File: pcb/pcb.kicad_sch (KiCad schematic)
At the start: 2 parts

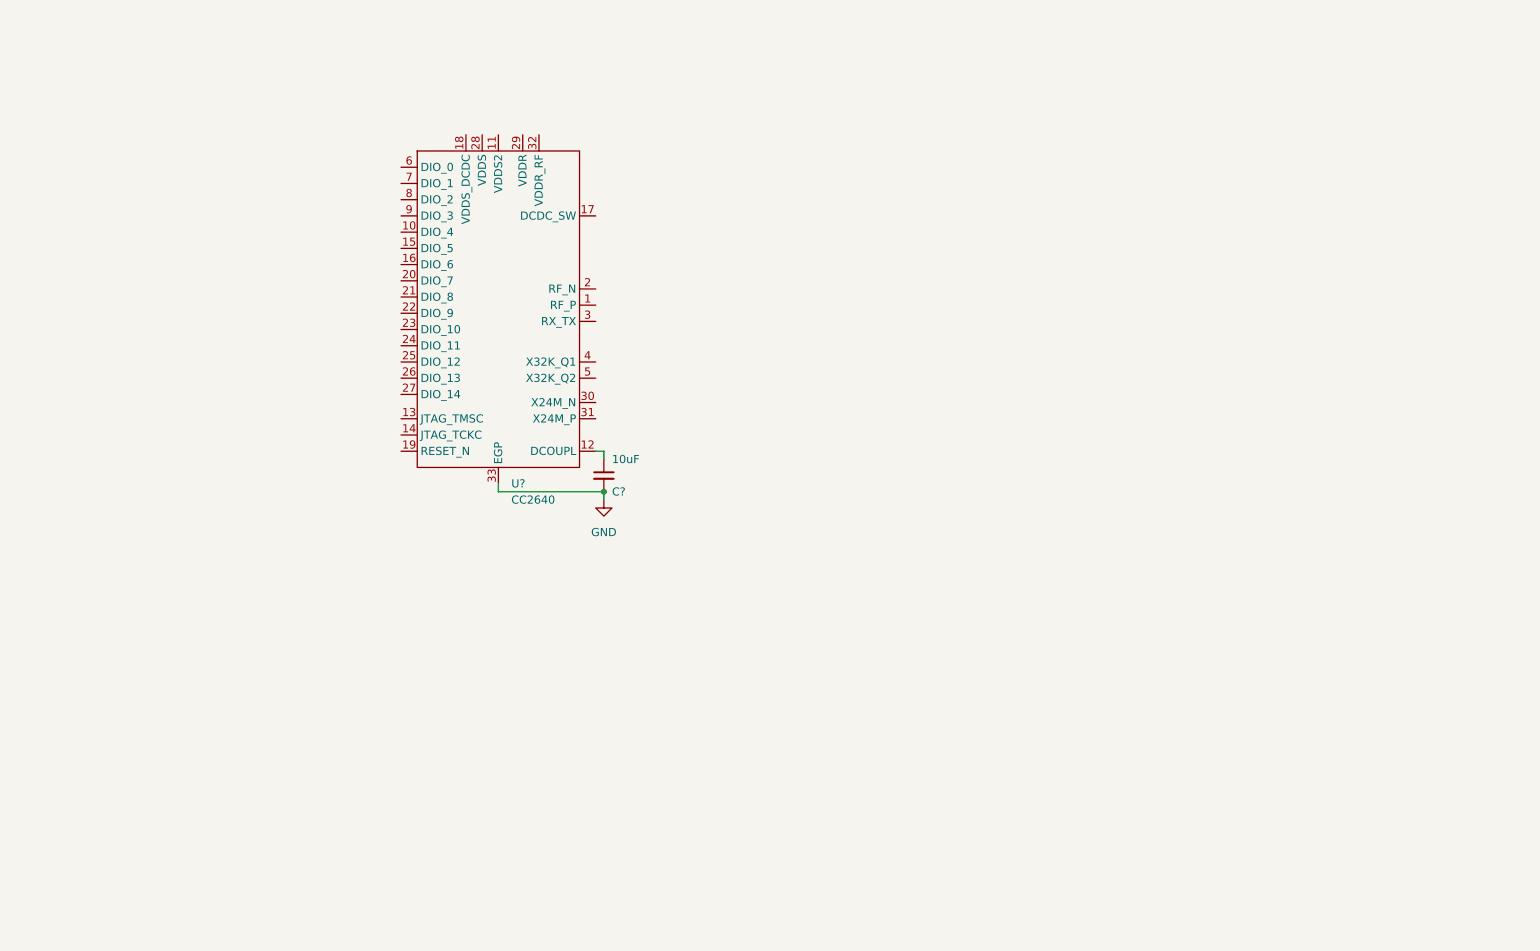
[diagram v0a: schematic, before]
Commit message: schematic
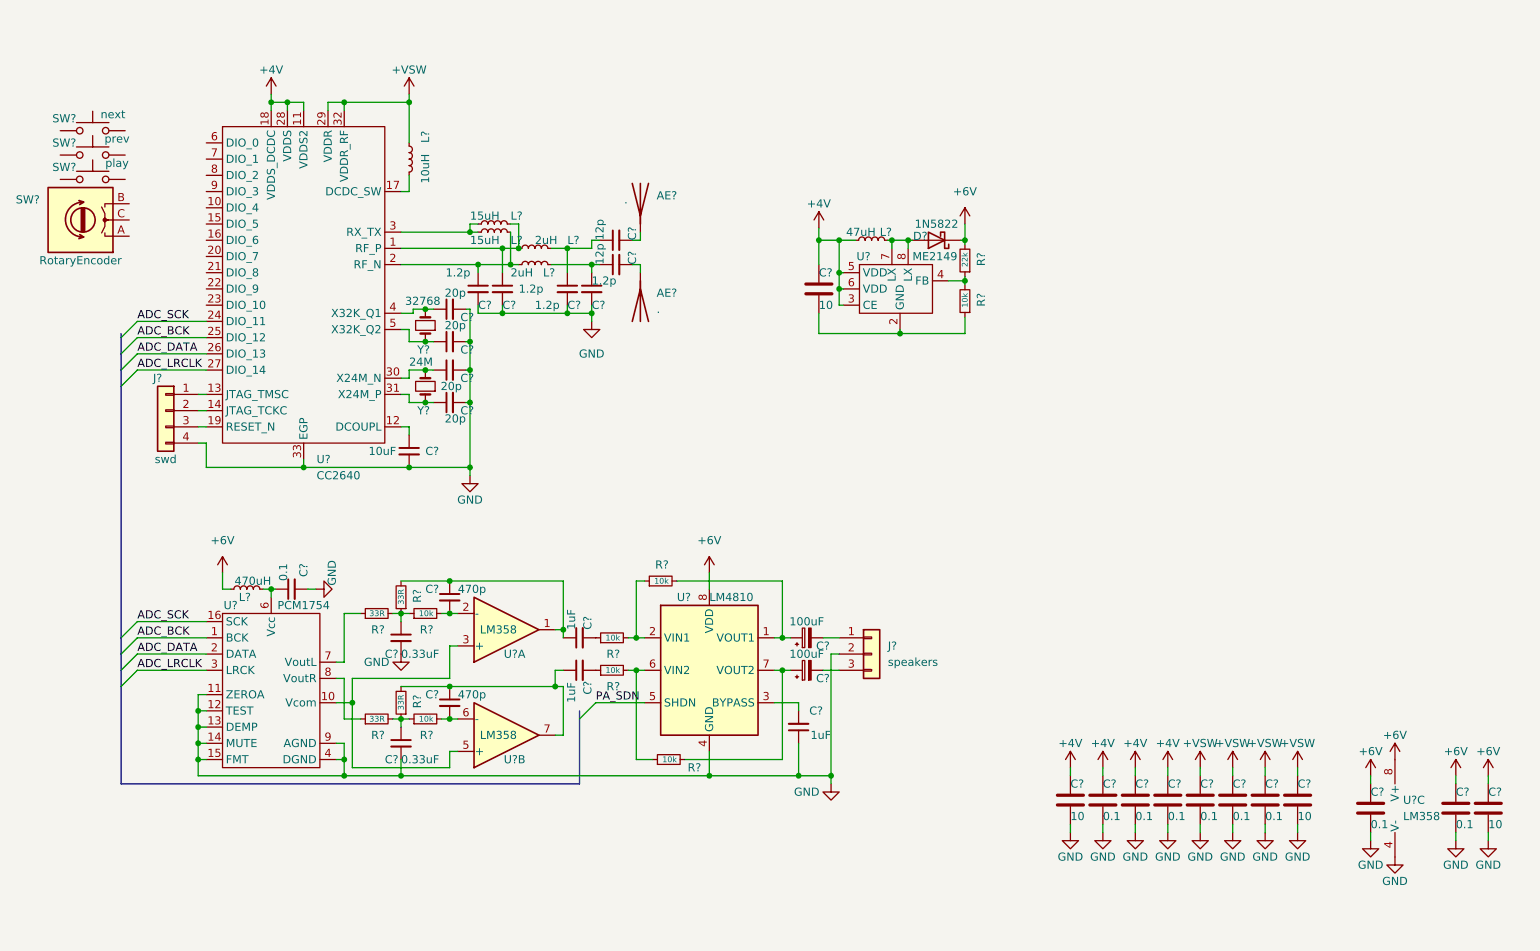
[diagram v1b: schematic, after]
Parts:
- added AE? (x2): ., symbol Device:Antenna
- added C? (x4): 1.2p, symbol Device:C_Small
- added C? (x2): 470p, symbol Device:C_Small
- added C? (x4): 20p, symbol Device:C_Small
- added C? (x8): 0.1, symbol Device:C
- added C? (x4): 10, symbol Device:C
- added C? (x2): 100uF, symbol Device:C_Polarized_Small
- added C? (x2): 12p, symbol Device:C_Small
- added C?: 0.1, symbol Device:C_Small
- added C? (x3): 1uF, symbol Device:C_Small
- added C? (x2): 0.33uF, symbol Device:C_Small
- added D?: 1N5822, symbol Device:D_Schottky
- added J?: speakers, symbol Connector_Generic:Conn_01x03
- added J?: swd, symbol Connector_Generic:Conn_01x04
- added L? (x2): 2uH, symbol Device:L_Small
- added L?: 47uH, symbol Device:L_Small
- added L? (x2): 15uH, symbol Device:L_Small
- added L?: 10uH, symbol Device:L_Small
- added L?: 470uH, symbol Device:L_Small
- added R? (x4): 33R, symbol Device:R_Small
- added R? (x7): 10k, symbol Device:R_Small
- added R?: 22k, symbol Device:R_Small
- added SW?: next, symbol Switch:SW_Push
- added SW?: play, symbol Switch:SW_Push
- added SW?: RotaryEncoder, symbol Device:RotaryEncoder
- added SW?: prev, symbol Switch:SW_Push
- added U? (x3): LM358, symbol Amplifier_Operational:LM358
- added U?: LM4810, Package_SO:TSSOP-8_3x3mm_P0.65mm, symbol Amplifier_Audio:LM4810
- added U?: PCM1754, symbol local:PCM1754
- added U?: ME2149, symbol local:ME2149
- added Y?: 24M, symbol Device:Crystal_Small
- added Y?: 32768, symbol Device:Crystal_Small
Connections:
- net GND: now also C?.1, C?.2, C?.2, C?.2, C?.2, C?.2, C?.2, C?.2, C?.2, C?.2, C?.2, C?.2, C?.2, C?.2, C?.2, C?.2, C?.2, C?.2, C?.2, C?.2, C?.2, C?.2, C?.2, J?.2 (Pin_2), J?.4 (Pin_4), U?.11 (ZEROA), U?.12 (TEST), U?.13 (DEMP), U?.14 (MUTE), U?.15 (FMT), U?.4 (DGND), U?.4 (GND), U?.4 (V-), U?.9 (AGND)
- net at U?.1 (RF_P): now also C?.1, L?.1, L?.2
- net +4V: now reaches U?.11 (VDDS2)
- net +4V: now also U?.18 (VDDS_DCDC), U?.28 (VDDS), C?.1, C?.1, C?.1, C?.1, C?.1, L?.1, U?.3 (CE), U?.5 (VDD), U?.6 (VDD)
- net at U?.13 (JTAG_TMSC): now also J?.1 (Pin_1)
- net at U?.14 (JTAG_TCKC): now also J?.2 (Pin_2)
- net at U?.17 (DCDC_SW): now also L?.2
- net at U?.19 (RESET_N): now also J?.3 (Pin_3)
- net at U?.2 (RF_N): now also C?.1, L?.1, L?.2
- net ADC_SCK: now reaches U?.24 (DIO_11)
- net ADC_SCK: now also U?.16 (SCK)
- net ADC_BCK: now reaches U?.25 (DIO_12)
- net ADC_BCK: now also U?.1 (BCK)
- net ADC_DATA: now reaches U?.26 (DIO_13)
- net ADC_DATA: now also U?.2 (DATA)
- net ADC_LRCLK: now reaches U?.27 (DIO_14)
- net ADC_LRCLK: now also U?.3 (LRCK)
- net +VSW: now reaches U?.29 (VDDR)
- net +VSW: now also U?.32 (VDDR_RF), C?.1, C?.1, C?.1, C?.1, L?.1
- net at U?.3 (RX_TX): now also L?.2, L?.2
- net at U?.30 (X24M_N): now also C?.1, Y?.2
- net at U?.31 (X24M_P): now also C?.1, Y?.1
- net at U?.4 (X32K_Q1): now also C?.1, Y?.2
- net at U?.5 (X32K_Q2): now also C?.1, Y?.1
- new net: R?.1, U?.8 (VoutR)
- new net: C?.1, R?.1, R?.1, R?.2 (x2)
- new net: C?.1, C?.1, L?.1 (x2)
- new net: C?.1, C?.1, R?.2, U?.7
- new net: C?.2, R?.2, U?.6 (-)
- new net: C?.2, R?.2, U?.2 (-)
- new net: C?.1, C?.1, R?.2, U?.1
- new net: U?.10 (Vcom), U?.3 (+), U?.5 (+)
- new net: R?.1, R?.2, U?.2 (VIN1)
- new net: C?.1, R?.2, U?.1 (VOUT1)
- new net: D?.2 (A), L?.2, U?.7 (LX), U?.8 (LX)
- new net: R?.1, R?.2, U?.6 (VIN2)
- new net: C?.1, R?.2, U?.7 (VOUT2)
- new net: C?.2, R?.1, U?.2 (GND)
- new net: R?.1, R?.2, U?.4 (FB)
- new net: AE?.1 (A), C?.2 (x2)
- new net: C?.2, J?.3 (Pin_3)
- new net: C?.2, J?.1 (Pin_1)
- new net: C?.2, R?.1 (x2)
- new net: C?.1, L?.2, U?.6 (Vcc)
- new net: C?.2, U?.3 (BYPASS)
- new net: R?.1, U?.7 (VoutL)
- new net +6V: C?.1, C?.1, C?.1, D?.1 (K), L?.1, R?.2, U?.8 (V+), U?.8 (VDD)
- new net PA_SDN: U?.5 (SHDN)
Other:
- moved on the sheet: C?, U?

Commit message: schematic png
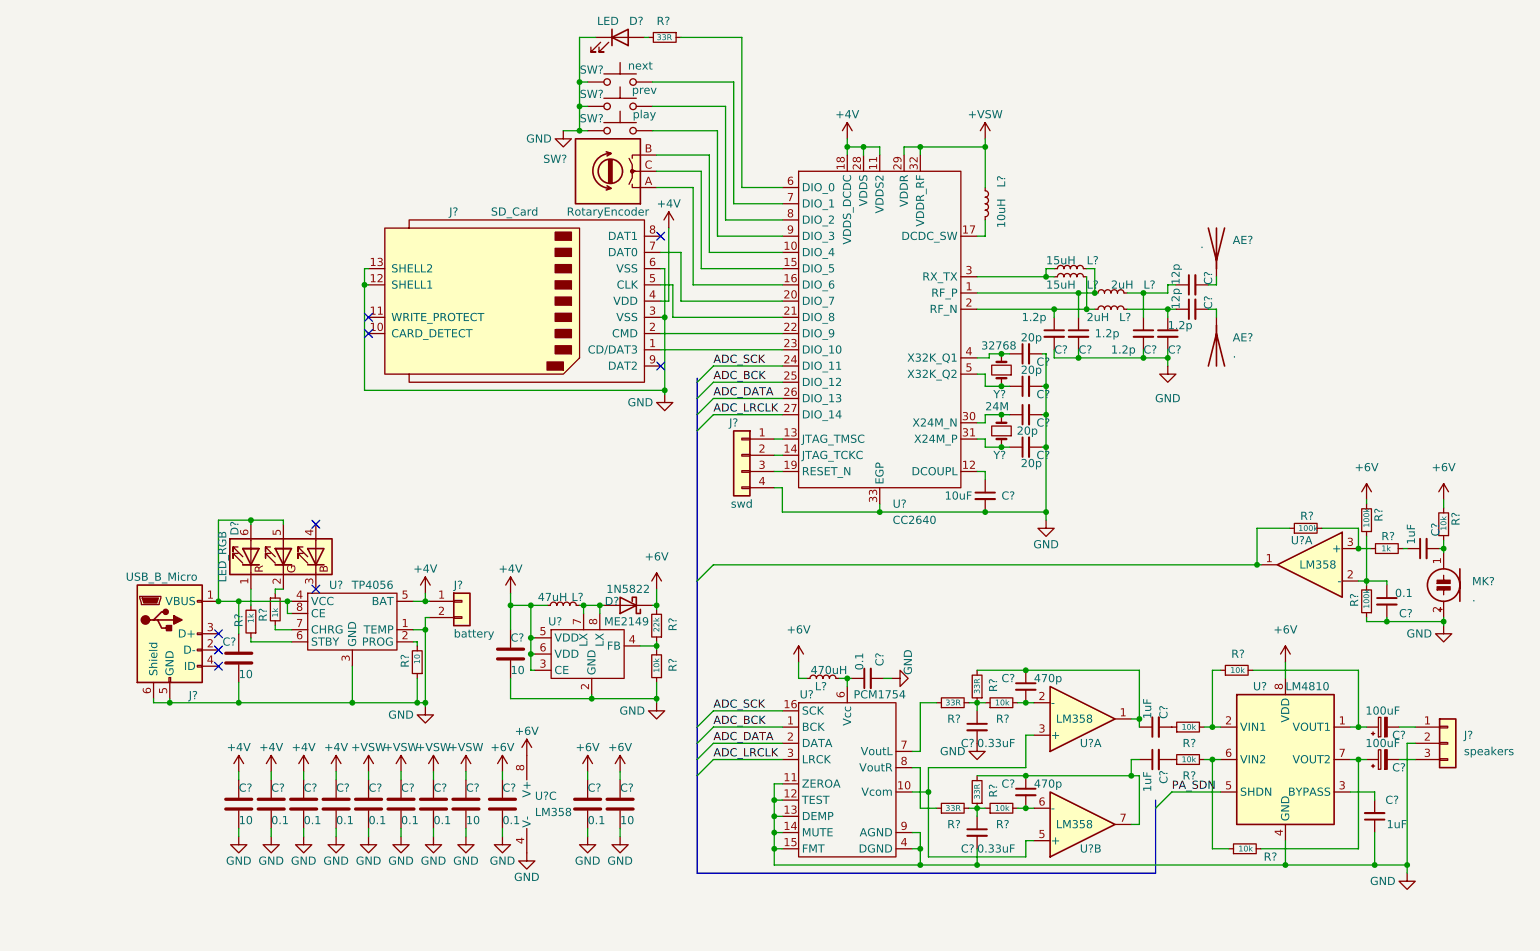
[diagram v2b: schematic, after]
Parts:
- added C?: 0.1, symbol Device:C_Small
- added C?: 10, symbol Device:C
- added C?: 1uF, symbol Device:C_Small
- added D?: LED, symbol Device:LED
- added D?: LED_RGB, symbol Device:LED_RGB
- added J?: SD_Card, symbol Connector:SD_Card
- added J?: USB_B_Micro, symbol Connector:USB_B_Micro
- added J?: battery, symbol Connector_Generic:Conn_01x02
- added MK?: ., symbol Device:Microphone_Condenser
- added R? (x3): 1k, symbol Device:R_Small
- added R? (x3): 100k, symbol Device:R_Small
- added R?: 10, symbol Device:R_Small
- added R?: 10k, symbol Device:R_Small
- added R?: 33R, symbol Device:R_Small
- added U?: TP4056, symbol local:TP4056
- added U?: LM358, symbol Amplifier_Operational:LM358
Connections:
- net +4V: now also J?.1 (Pin_1), J?.4 (VDD), U?.5 (BAT)
- net +6V: now also R?.2, R?.2
- net GND: now also C?.2, R?.1, SW?.1, SW?.1, SW?.1, U?.2 (GND), C?.2, C?.2, D?.1 (K), J?.12 (SHELL1), J?.13 (SHELL2), J?.2 (Pin_2), J?.3 (VSS), J?.5 (GND), J?.6 (Shield), J?.6 (VSS), MK?.2 (+), R?.1, R?.1, U?.1 (TEMP), U?.3 (GND)
- net at SW?.2: now also U?.7 (DIO_1)
- net at U?.10 (DIO_4): now also SW?.B
- net at U?.15 (DIO_5): now also SW?.C
- net at U?.16 (DIO_6): now also SW?.A
- net at U?.20 (DIO_7): now also J?.7 (DAT0)
- net at U?.21 (DIO_8): now also J?.5 (CLK)
- net at U?.22 (DIO_9): now also J?.2 (CMD)
- net at U?.23 (DIO_10): now also J?.1 (CD/DAT3)
- net at U?.6 (DIO_0): now also R?.1
- net at U?.8 (DIO_2): now also SW?.2
- net at U?.9 (DIO_3): now also SW?.2
- new net: R?.1, R?.2, U?.3 (+)
- new net: C?.1, R?.2
- new net: D?.2 (A), R?.2
- new net: C?.1, R?.1, R?.2, U?.2 (-)
- new net: R?.2, U?.2 (PROG)
- new net: C?.2, MK?.1 (-), R?.1
- new net: C?.1, D?.5 (GA), D?.6 (RA), J?.1 (VBUS), U?.4 (VCC), U?.8 (CE)
- new net: R?.1, U?.6 (STBY)
- new net: R?.2, U?.7 (CHRG)
- new net: D?.1 (RK), R?.2
- new net: D?.2 (GK), R?.1
- new net: R?.1, U?.1
- no-connect marks 0 -> 9
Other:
- moved on the sheet: AE?, C?, D?, J?, L?, R?, SW?, U?, U?A, U?B, U?C, Y?

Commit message: pcb footprints
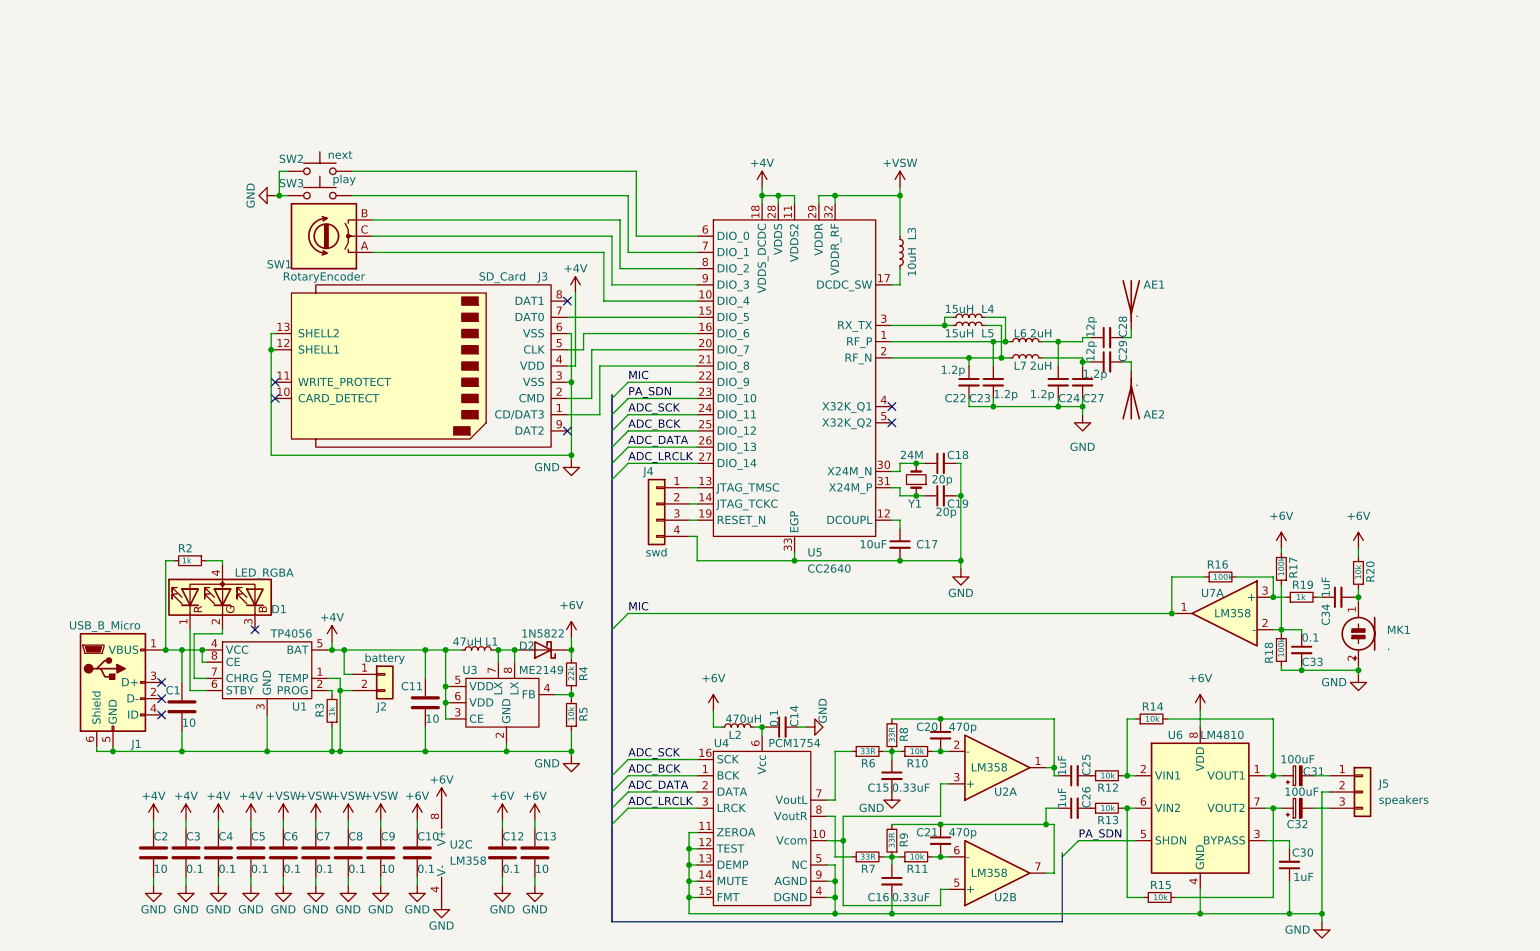
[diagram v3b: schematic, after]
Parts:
- removed C? (x2): 20p, symbol Device:C_Small
- removed D?: LED, symbol Device:LED
- removed D?: LED_RGB, symbol Device:LED_RGB
- removed R?: 1k, symbol Device:R_Small
- removed R?: 33R, symbol Device:R_Small
- removed SW?: prev, symbol Switch:SW_Push
- removed Y?: 32768, symbol Device:Crystal_Small
- added D1: LED_RGBA, LED_SMD:LED_Cree-PLCC4_3.2x2.8mm_CCW, symbol Device:LED_RGBA
- AE1, AE2: renamed from AE?; footprint (none) -> Connector_Wire:SolderWirePad_1x01_SMD_1x2mm
- C1, C11, C13, C17, C2, C25, C26, C30, C34, C9: renamed from C?; footprint (none) -> Capacitor_SMD:C_0805_2012Metric
- C10, C12, C14, C18, C19, C3, C33, C4, C5, C6, C7, C8: renamed from C?; footprint (none) -> Capacitor_SMD:C_0402_1005Metric
- C15, C16, C20, C21, C22, C23, C24, C27, C28, C29: renamed from C?; footprint (none) -> Capacitor_SMD:C_0603_1608Metric
- C31, C32: renamed from C?; footprint (none) -> Capacitor_Tantalum_SMD:CP_EIA-1608-08_AVX-J
- D2: renamed from D?; footprint (none) -> Diode_SMD:D_SMA
- J1: renamed from J?; footprint (none) -> Connector_USB:USB_Micro-B_Amphenol_10104110_Horizontal
- J2: renamed from J?; footprint (none) -> Connector_PinHeader_2.54mm:PinHeader_1x02_P2.54mm_Vertical
- J3: renamed from J?; footprint (none) -> Connector_Card:SD_Hirose_DM1AA_SF_PEJ82
- J4: renamed from J?; footprint (none) -> Connector_PinHeader_1.00mm:PinHeader_1x04_P1.00mm_Vertical_SMD_Pin1Left
- J5: renamed from J?; footprint (none) -> Connector_PinHeader_2.54mm:PinHeader_1x03_P2.54mm_Vertical
- L1, L2, L3, L4, L5, L6, L7: renamed from L?; footprint (none) -> Inductor_SMD:L_0603_1608Metric
- MK1: renamed from MK?; footprint (none) -> Capacitor_THT:CP_Radial_D5.0mm_P2.50mm
- R10, R11, R12, R13, R14, R15, R16, R17, R18, R19, R2, R20, R5, R6, R7, R8, R9: renamed from R?; footprint (none) -> Resistor_SMD:R_0402_1005Metric
- R3: renamed from R?; value 10 -> 1k; footprint (none) -> Resistor_SMD:R_0402_1005Metric
- R4: renamed from R?; footprint (none) -> Resistor_SMD:R_0805_2012Metric
- SW1: renamed from SW?; footprint (none) -> local:mouse_encoder
- SW2, SW3: renamed from SW?; footprint (none) -> Button_Switch_THT:SW_PUSH_6mm
- U1: renamed from U?; footprint (none) -> Package_SO:SOP-8_3.9x4.9mm_P1.27mm
- U2, U7: renamed from U?; footprint (none) -> Package_SO:SOIC-8_3.9x4.9mm_P1.27mm
- U3: renamed from U?; footprint (none) -> Package_SO:SOIC-8-N7_3.9x4.9mm_P1.27mm
- U4: renamed from U?; footprint (none) -> Package_SO:SSOP-16_5.3x6.2mm_P0.65mm
- U5: renamed from U?; footprint (none) -> Package_DFN_QFN:HVQFN-32-1EP_5x5mm_P0.5mm_EP3.1x3.1mm
- Y1: renamed from Y?; footprint (none) -> Crystal:Crystal_SMD_5032-2Pin_5.0x3.2mm
- gave numbers to parts that had none: 1
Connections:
- net GND: now also U4.5 (NC)
- net PA_SDN: now also U5.23 (DIO_10)
- net at SW2.2: now also U5.6 (DIO_0); no longer U5.7 (DIO_1)
- net at J3.1 (CD/DAT3): now also U5.21 (DIO_8); no longer U5.23 (DIO_10)
- net at J3.2 (CMD): now also U5.20 (DIO_7); no longer U5.22 (DIO_9)
- net at J3.5 (CLK): now also U5.16 (DIO_6); no longer U5.21 (DIO_8)
- net at J3.7 (DAT0): now also U5.15 (DIO_5); no longer U5.20 (DIO_7)
- net at U5.10 (DIO_4): now also SW1.A; no longer SW1.B
- net at SW1.C: now also U5.9 (DIO_3); no longer U5.15 (DIO_5)
- net at U5.8 (DIO_2): now also SW1.B
- net at SW3.2: now also U5.7 (DIO_1); no longer U5.9 (DIO_3)
- net at C1.1, J1.1 (VBUS), U1.4 (VCC)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: now also R2.2
- net at U1.6 (STBY): now also D1.1 (RK)
- net at U1.7 (CHRG): now also D1.2 (GK); no longer R2.2
- net at R2.1: now also D1.4 (A)
- net MIC: now reaches R16.1, U7.1
- net MIC: now also U5.22 (DIO_9)
- no-connect marks 9 -> 10
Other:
- moved on the sheet: AE1, AE2, C1, C10, C11, C12, C13, C14, C15, C16, C17, C18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
